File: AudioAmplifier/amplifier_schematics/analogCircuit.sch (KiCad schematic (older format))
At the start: 3 parts

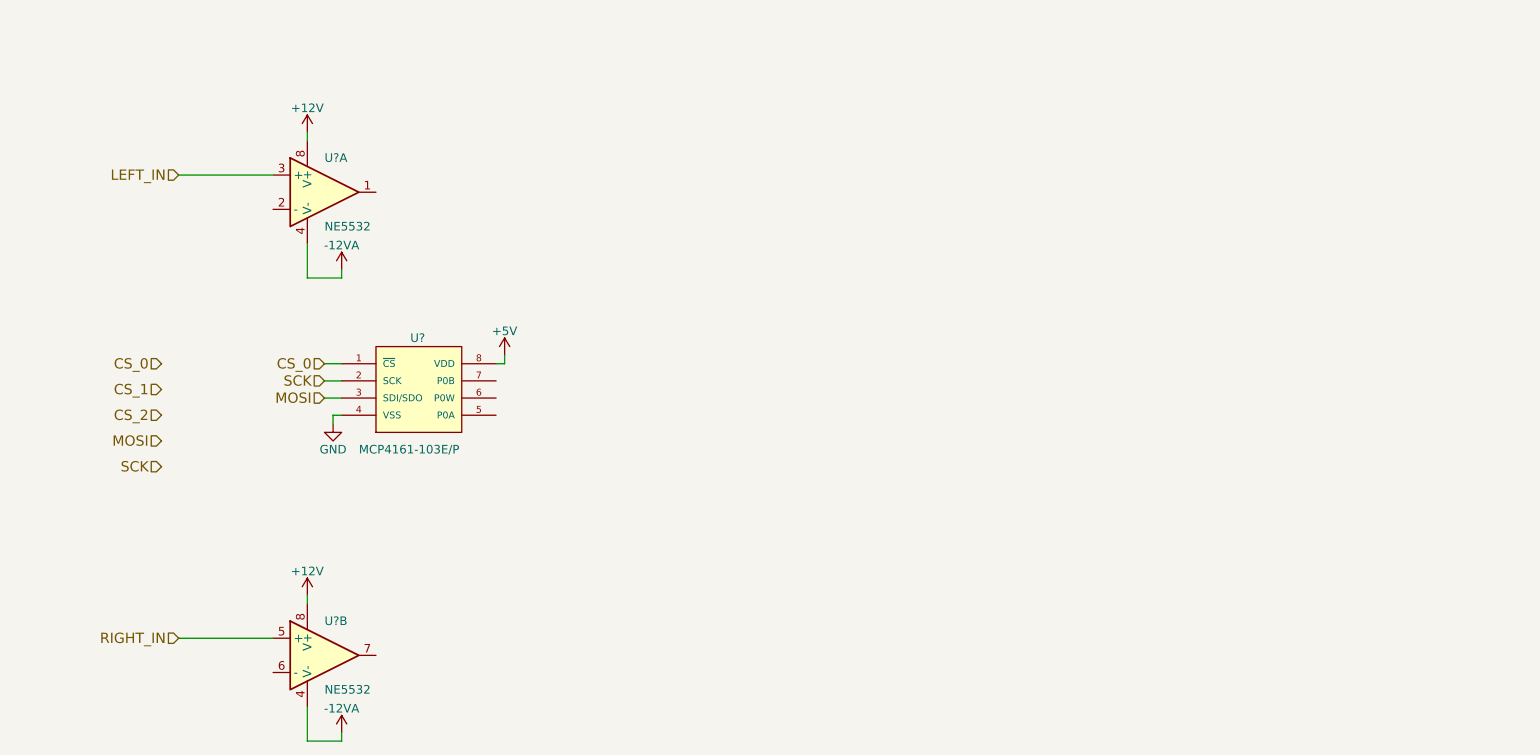
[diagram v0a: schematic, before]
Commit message: kicad
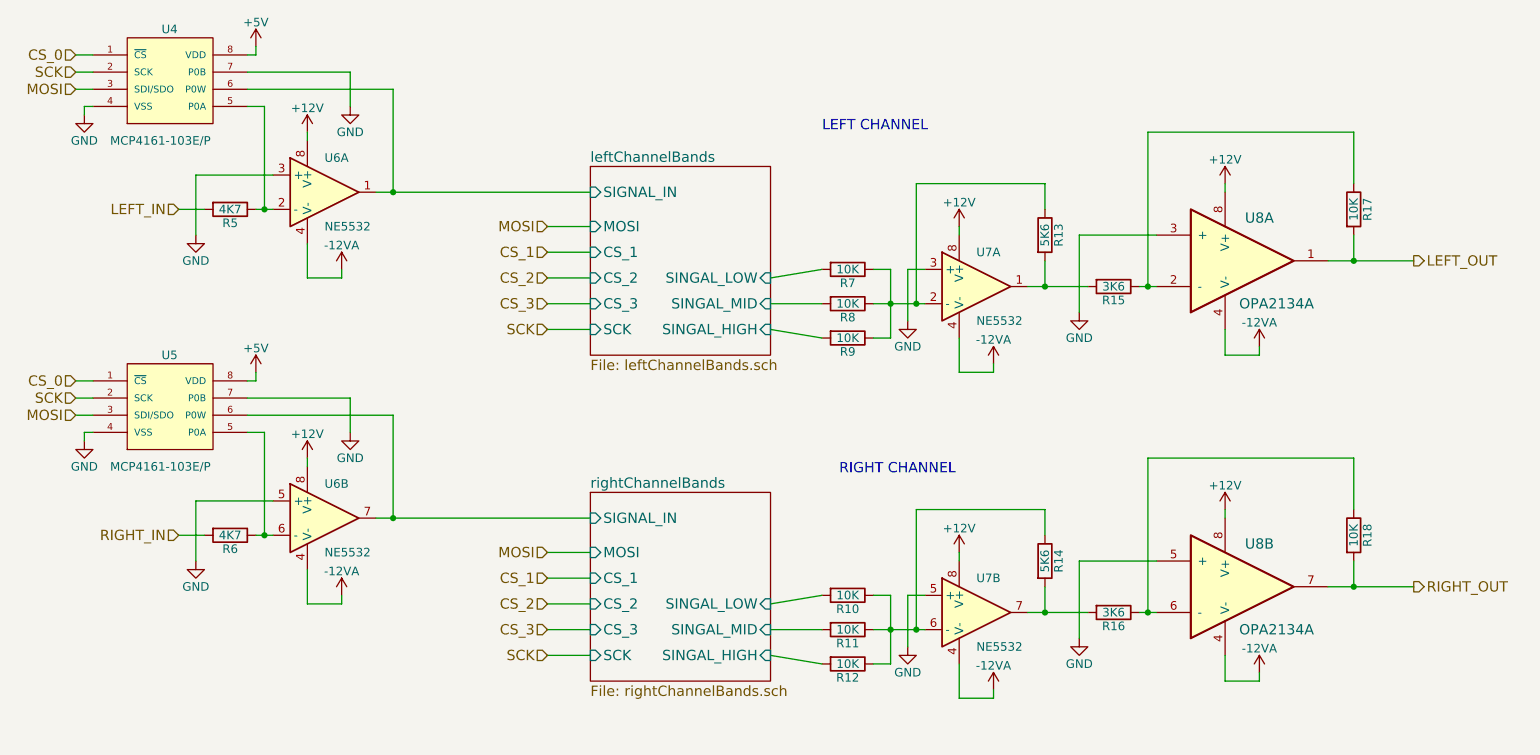
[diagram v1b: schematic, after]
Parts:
- added R10, R11, R12, R17, R18, R7, R8, R9: 10K, Resistors_THT:R_Axial_DIN0207_L6.3mm_D2.5mm_P10.16mm_Horizontal, symbol R
- added R13, R14: 5K6, Resistors_THT:R_Axial_DIN0207_L6.3mm_D2.5mm_P10.16mm_Horizontal, symbol R
- added R15, R16: 3K6, Resistors_THT:R_Axial_DIN0207_L6.3mm_D2.5mm_P10.16mm_Horizontal, symbol R
- added R5, R6: 4K7, Resistors_THT:R_Axial_DIN0207_L6.3mm_D2.5mm_P10.16mm_Horizontal, symbol R
- added U5: MCP4161-103E/P, Don-Fet-driver:DIP254P762X533-8, symbol MCP4161-103E/P
- added U7: NE5532, Don-Fet-driver:DIP254P762X533-8, symbol NE5532
- added U8: OPA2134A, Don-Fet-driver:DIP254P762X533-8, symbol OPA2134A
- U4: renamed from U?; footprint DIP254P762X533-8 -> Don-Fet-driver:DIP254P762X533-8
- U6: renamed from U?; footprint (none) -> Don-Fet-driver:DIP254P762X533-8
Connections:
- net +12V: now also U7.8 (V+), U7.8 (V+), U8.8 (V+), U8.8 (V+)
- net +5V: now also U5.8 (VDD)
- net -12VA: now also U7.4 (V-), U7.4 (V-), U8.4 (V-), U8.4 (V-)
- net CS_0: now also U5.1 (~CS)
- net GND: now also U4.7 (P0B), U6.3 (+), U6.5 (+), U5.4 (VSS), U5.7 (P0B), U7.3 (+), U7.5 (+), U8.3 (+), U8.5 (+)
- net LEFT_IN: now also R5.2; no longer U6.3 (+)
- net MOSI: now also U5.3 (SDI/SDO)
- net RIGHT_IN: now also R6.2; no longer U6.5 (+)
- net SCK: now also U5.2 (SCK)
- net leftChannelBands/SIGNAL_IN: now reaches U6.1
- net leftChannelBands/SIGNAL_IN: now also U4.6 (P0W)
- net at U6.2 (-): now also U4.5 (P0A), R5.1
- net at U6.6 (-): now also R6.1, U5.5 (P0A)
- net rightChannelBands/SIGNAL_IN: now reaches U6.7
- net rightChannelBands/SIGNAL_IN: now also U5.6 (P0W)
- new net: R13.1, R7.1, R8.1, R9.1, U7.2 (-)
- new net: R13.2, R15.2, U7.1
- new net: R10.1, R11.1, R12.1, R14.1, U7.6 (-)
- new net: R14.2, R16.2, U7.7
- new net: R15.1, R17.1, U8.2 (-)
- new net: R16.1, R18.1, U8.6 (-)
- new net LEFT_OUT: R17.2, U8.1
- new net RIGHT_OUT: R18.2, U8.7
- new net leftChannelBands/SINGAL_HIGH: R9.2
- new net leftChannelBands/SINGAL_LOW: R7.2
- new net leftChannelBands/SINGAL_MID: R8.2
- new net rightChannelBands/SINGAL_HIGH: R12.2
- new net rightChannelBands/SINGAL_LOW: R10.2
- new net rightChannelBands/SINGAL_MID: R11.2
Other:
- note added: "LEFT CHANNEL"
- note added: "RIGHT CHANNEL"
- moved on the sheet: U4, U6B
